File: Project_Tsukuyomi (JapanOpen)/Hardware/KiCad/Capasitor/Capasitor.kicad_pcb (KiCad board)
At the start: 2 copper layers, 106 x 13 mm, 9 parts, among them J1 Conn_01x02_Socket

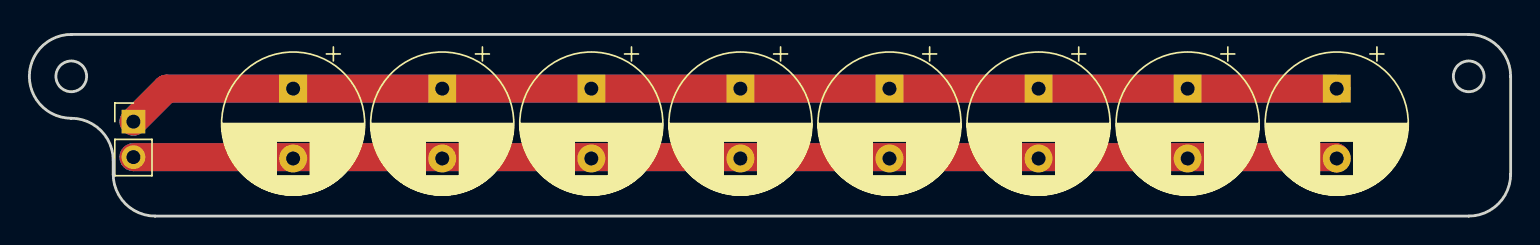
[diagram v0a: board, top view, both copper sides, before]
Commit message: 溜まった変更大放出
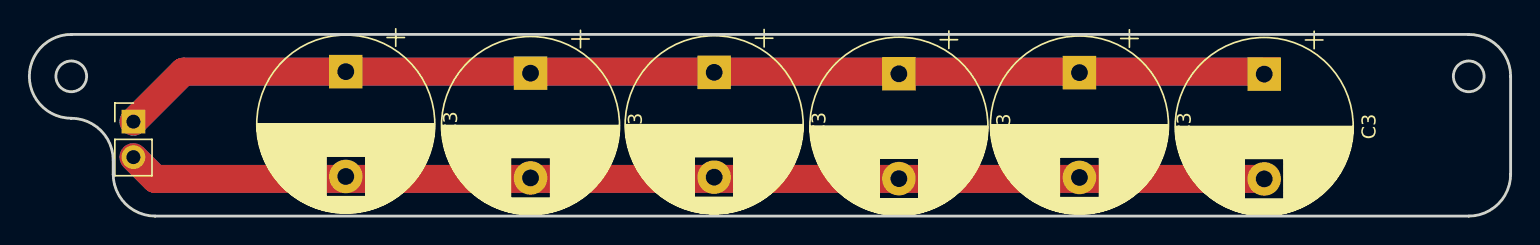
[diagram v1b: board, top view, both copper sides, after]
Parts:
- removed C1, C2, C4, C5, C6, C8, C9: C, Capacitor_THT:CP_Radial_D10.0mm_P5.00mm
- added C3: C, Capacitor_THT:CP_Radial_D12.5mm_P7.50mm, F.Cu at (172.1, 97.8)
- added C3: C, Capacitor_THT:CP_Radial_D12.5mm_P7.50mm, F.Cu at (132.8, 97.9)
- added C3: C, Capacitor_THT:CP_Radial_D12.5mm_P7.50mm, F.Cu at (185.3, 97.9)
- added C3: C, Capacitor_THT:CP_Radial_D12.5mm_P7.50mm, F.Cu at (159.2, 97.9)
- added C3: C, Capacitor_THT:CP_Radial_D12.5mm_P7.50mm, F.Cu at (145.9, 97.8)
- C3: footprint Capacitor_THT:CP_Radial_D10.0mm_P5.00mm -> Capacitor_THT:CP_Radial_D12.5mm_P7.50mm
- moved C3 3.96 mm to (119.6, 97.8)
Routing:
- net Net-(J1-Pin_1): track 174.2 -> 164.9 mm
- net Net-(J1-Pin_2): track 172.3 -> 163.1 mm
